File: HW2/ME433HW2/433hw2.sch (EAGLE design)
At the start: 1 part

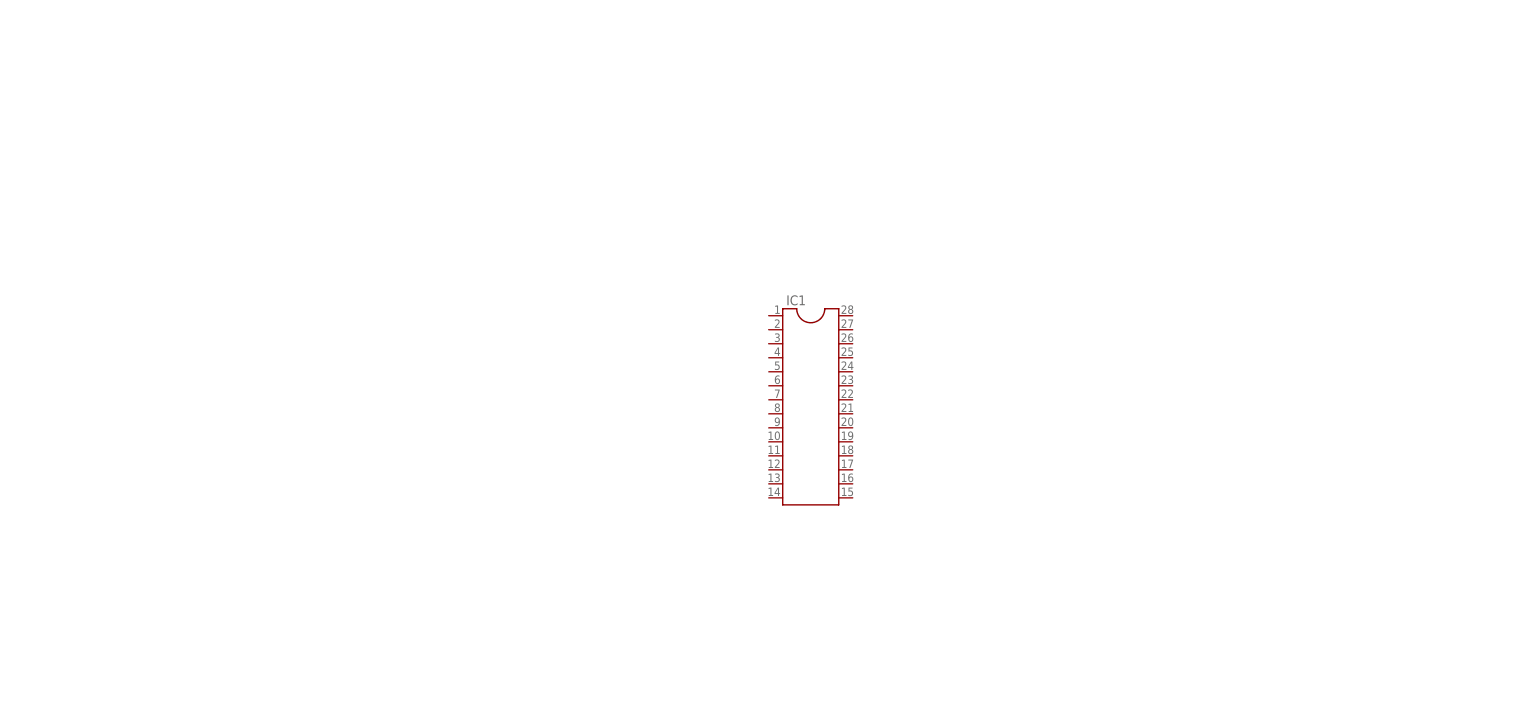
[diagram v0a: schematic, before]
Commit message: SCHEMATIC
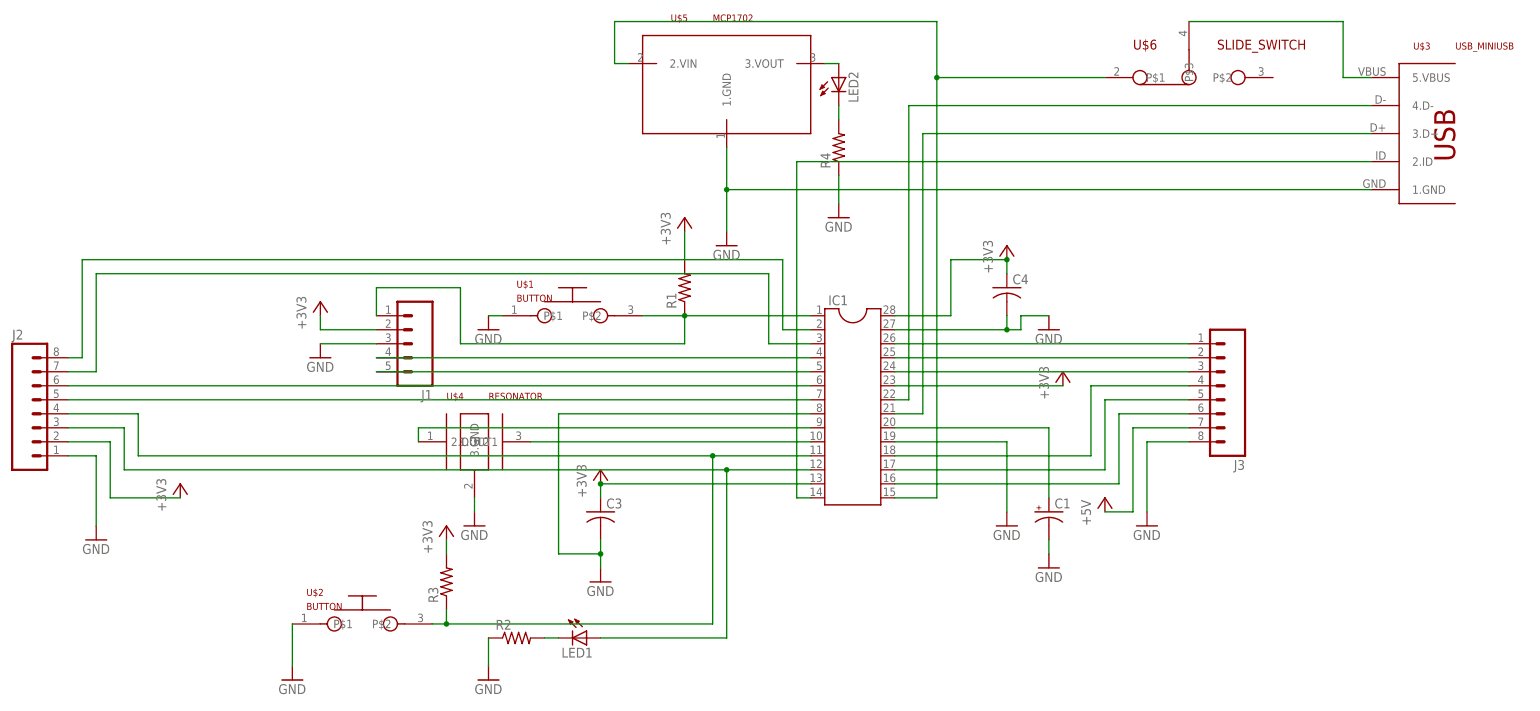
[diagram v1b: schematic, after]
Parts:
- added C1: (no value), 433LIB:CPOL-USE2.5-6
- added C3, C4: (no value), 433LIB:C-US025-025X050
- added J1: (no value), 433LIB:M05PTH
- added J2, J3: (no value), 433LIB:M08
- added LED1, LED2: (no value), 433LIB:LED3MM
- added R1, R2, R3, R4: (no value), 433LIB:R-US_0207/7
- added U$1, U$2: BUTTON, 433LIB:BUTTON
- added U$3: USB_MINIUSB, 433LIB:USB_MINIUSB
- added U$4: RESONATOR, 433LIB:RESONATOR
- added U$5: MCP1702, 433LIB:MCP1702
- added U$6: SLIDE_SWITCH, 433LIB:SLIDE_SWITCH
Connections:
- new net +3V3: C3.1, C4.1, IC1.13, IC1.23, IC1.28, J1.2, J2.2, R1.2, R3.2
- new net +5V: J3.7
- new net GND: C1.-, C3.2, C4.2, IC1.19, IC1.27, IC1.8, J1.3, J2.1, J3.8, R2.1, R4.1, U$1.P$1, U$2.P$1, U$3.1.GND, U$4.3.GND, U$5.1.GND
- new net N$1: IC1.1, J1.1, R1.1, U$1.P$2
- new net N$10: IC1.15, U$5.2.VIN, U$6.P$1
- new net N$11: C1.+, IC1.20
- new net N$12: IC1.14, U$3.2.ID
- new net N$13: IC1.22, U$3.4.D-
- new net N$14: IC1.21, U$3.3.D+
- new net N$15: IC1.2, J2.8
- new net N$16: IC1.26, J3.1
- new net N$17: IC1.11, J2.4, R3.1, U$2.P$2
- new net N$18: IC1.3, J2.7
- new net N$19: IC1.6, J2.6
- new net N$2: IC1.10, U$4.2.OUT2
- new net N$20: IC1.7, J2.5
- new net N$21: IC1.25, J3.2
- new net N$22: IC1.24, J3.3
- new net N$23: IC1.18, J3.4
- new net N$24: IC1.17, J3.5
- new net N$25: IC1.16, J3.6
- new net N$26: U$3.5.VBUS, U$6.P$3
- new net N$3: IC1.9, U$4.1.OUT1
- new net N$4: IC1.5, J1.5
- new net N$5: LED1.C, R2.2
- new net N$6: IC1.12, J2.3, LED1.A
- new net N$7: IC1.4, J1.4
- new net N$8: LED2.A, U$5.3.VOUT
- new net N$9: LED2.C, R4.2
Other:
- moved on the sheet: IC1
